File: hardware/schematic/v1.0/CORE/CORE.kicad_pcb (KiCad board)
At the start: 2 copper layers, 1 x 9 mm, 89 parts, among them J1 Conn_01x16_Socket, J10 USB_C_Receptacle_USB2.0_16P, J11 Conn_01x06_Socket, J12 Conn_01x16_Socket, J2 Conn_Coaxial, J3 Conn_Coaxial, J4 Conn_Coaxial, J5 Conn_Coaxial, J6 Conn_Coaxial, J7 Conn_Coaxial, J8 Conn_Coaxial, J9 Conn_Coaxial, M1 ZYNQ7010&7020, U1 TXS02612RTWR, U2 TPS78633, U3 SD_Card, U4 AMS1117-2.5, U5 AMS1117-1.8, U6 CH340E, U7 TPS78633

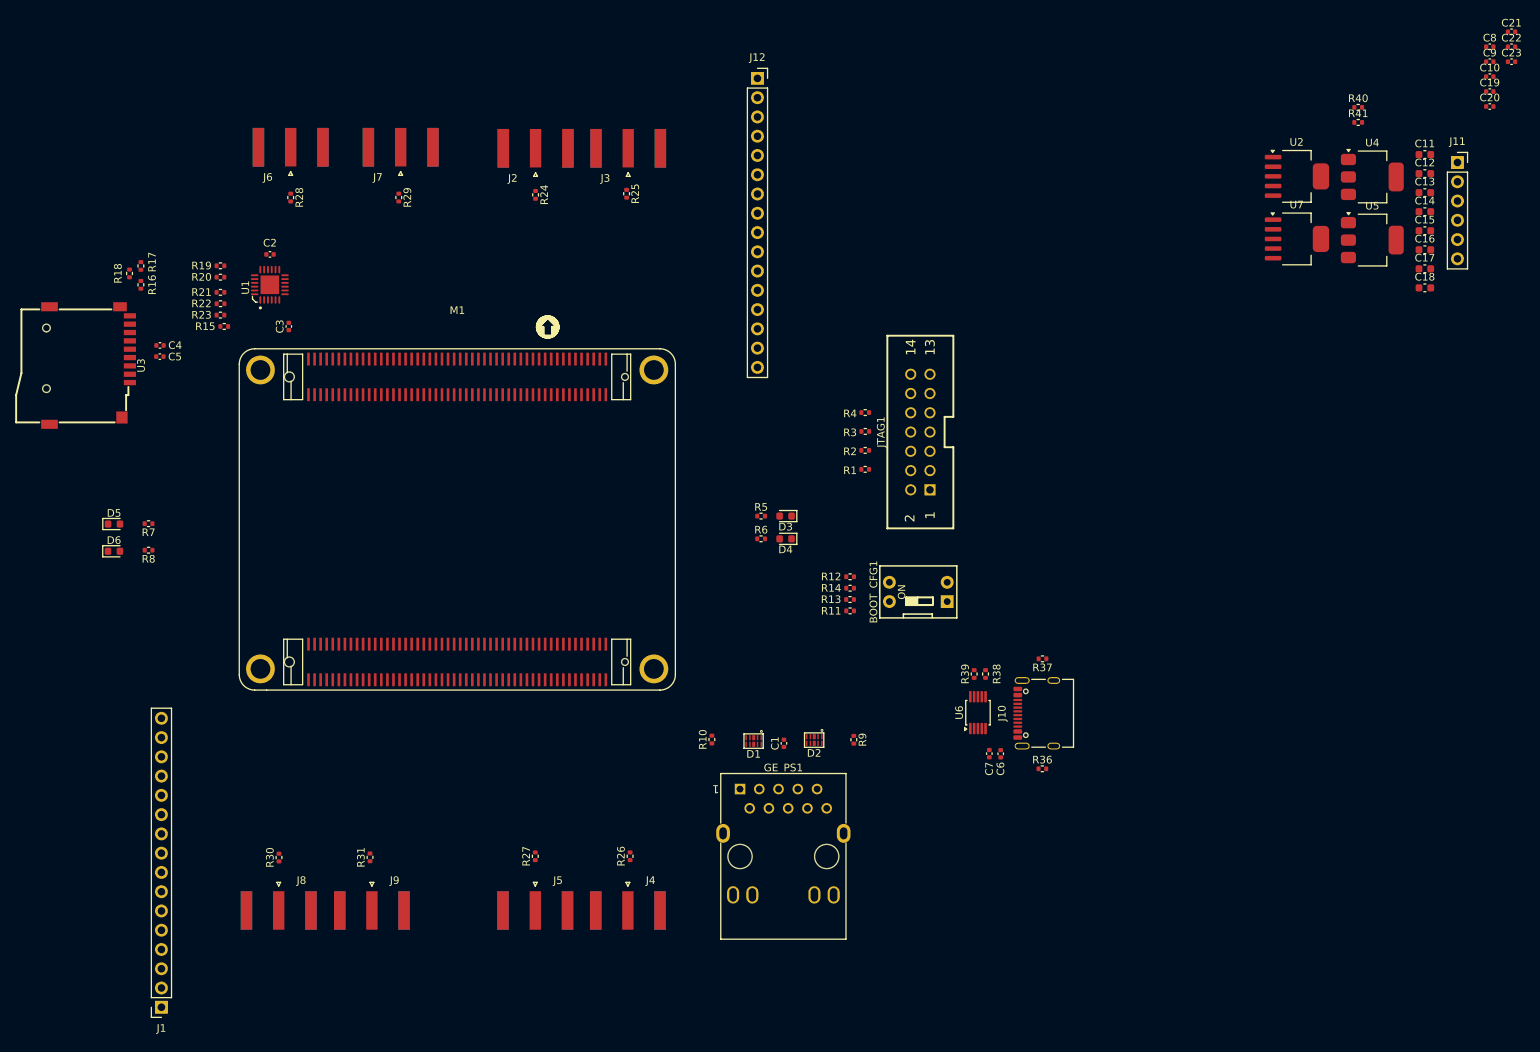
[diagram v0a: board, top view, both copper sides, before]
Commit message: sch update
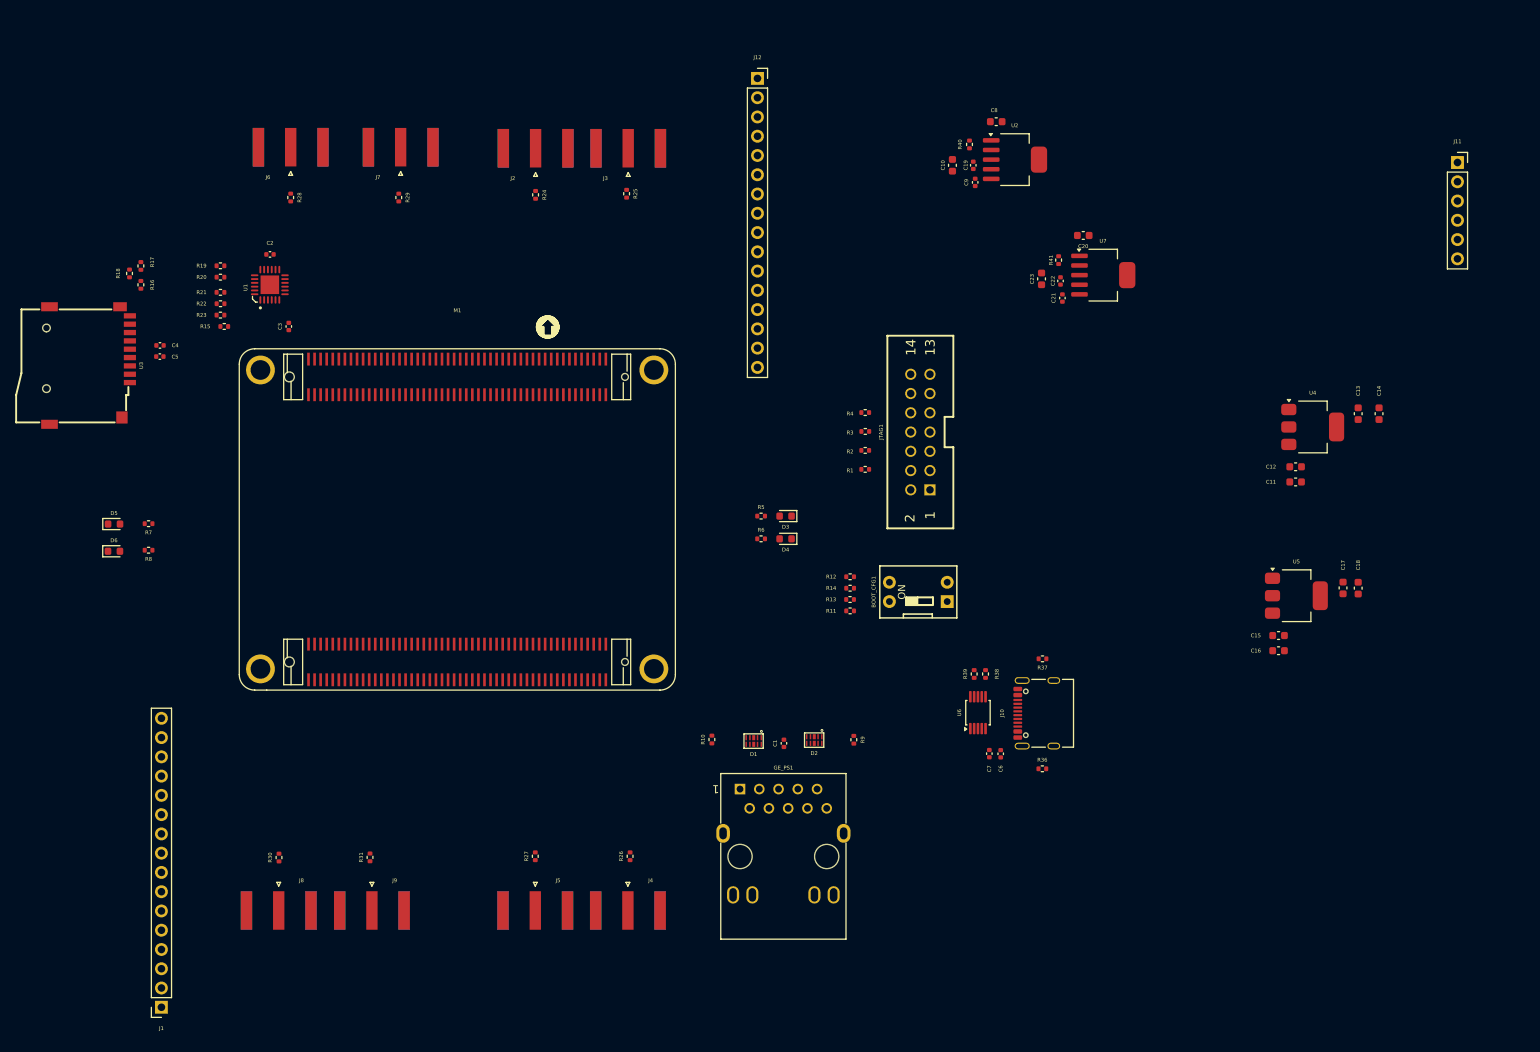
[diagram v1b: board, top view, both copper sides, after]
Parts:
- C10, C23: value 1uF -> 10uF; footprint Capacitor_SMD:C_0402_1005Metric -> Capacitor_SMD:C_0603_1608Metric
- C11, C15: value 4.7uF -> 10uF
- C20, C8: value 2.2uF -> 10uF; footprint Capacitor_SMD:C_0402_1005Metric -> Capacitor_SMD:C_0603_1608Metric
- moved C10 71.8 mm to (195.0, 49.2), turned to -90 degrees
- moved C9 69.7 mm to (198.0, 51.5), turned to 90 degrees
- moved C21 68.8 mm to (209.5, 66.8), turned to 90 degrees
- moved C19 68.8 mm to (197.8, 49.2), turned to -90 degrees
- moved C23 68.3 mm to (206.8, 64.2), turned to -90 degrees
- moved C22 67.0 mm to (209.2, 64.5), turned to -90 degrees
- moved C8 65.8 mm to (200.8, 43.5), turned to 180 degrees
- moved C15 56.7 mm to (238.0, 111.2)
- moved C16 56.3 mm to (238.0, 113.2)
- moved C20 56.2 mm to (212.2, 58.5), turned to 180 degrees
- moved R40 51.5 mm to (197.2, 46.5), turned to -90 degrees
- moved U5 47.9 mm to (240.3, 106.0)
- moved C11 46.4 mm to (240.2, 91.0)
- moved R41 43.5 mm to (209.0, 61.8), turned to -90 degrees
- moved C17 43.4 mm to (246.5, 105.0), turned to 90 degrees
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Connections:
- C11 pad 1: +5V -> +3.3V
- C12 pad 1: +5V -> +3.3V
- C15 pad 1: +5V -> +3.3V
- C16 pad 1: +5V -> +3.3V
- M1 pad J2_83: unconnected-(M1-83-PadJ2_83) -> XADC_VP
- M1 pad J2_85: unconnected-(M1-85-PadJ2_85) -> XADC_VN
- U4 pad 3: +5V -> +3.3V
- U5 pad 3: +5V -> +3.3V
